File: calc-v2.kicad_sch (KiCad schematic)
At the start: 110 parts, among them IC1 ISL91107IRTNZ-T, J1 USB_C_Receptacle_USB2.0_16P, J2 Conn_01x02_MountingPin, SW1 SW_Push_45deg, SW10 SW_Push_45deg, SW11 SW_Push_45deg, SW12 SW_Push_45deg, SW13 SW_Push_45deg, SW14 SW_Push_45deg, SW15 SW_Push_45deg, SW16 SW_Push_45deg, SW17 SW_Push_45deg, SW18 SW_Push_45deg, SW19 SW_Push_45deg, SW2 SW_Push_45deg, SW20 SW_Push_45deg, SW21 SW_Push_45deg, SW22 SW_Push_45deg, SW23 SW_Push_45deg, SW24 SW_Push_45deg, SW25 SW_Push_45deg, SW26 SW_Push_45deg, SW27 SW_Push_45deg, SW28 SW_Push_45deg, SW29 SW_Push_45deg, SW3 SW_Push_45deg, SW30 SW_Push_45deg, SW31 SW_Push_45deg, SW32 SW_Push_45deg, SW33 SW_Push_45deg, SW34 SW_Push_45deg, SW35 SW_Push_45deg, SW36 SW_Push_45deg, SW37 SW_Push_45deg, SW38 SW_Push_45deg, SW39 SW_Push_45deg, SW4 SW_Push_45deg, SW40 SW_Push_45deg, SW41 SW_Push_45deg, SW42 SW_Push_45deg, SW43 SW_Push_45deg, SW44 SW_Push_45deg, SW45 SW_Push_45deg, SW46 SW_Push_45deg, SW47 SW_Push_45deg, SW48 SW_Push_45deg, SW49 SW_Push_45deg, SW5 SW_Push_45deg, SW6 SW_Push_45deg, SW7 SW_Push_45deg, SW8 SW_Push_45deg, SW9 SW_Push_45deg, U1 W25Q128JVS, U3 BQ24074RGT, U4 TPS61165DBV, U5 RP2350B, U6 APS6404L-3SQRx-ZR, Y1 ABM8-272-T3

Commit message: screen, moving buttons
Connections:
- net GND: now also DS1.3 (IM0), DS1.34 (DOTCLK), DS1.35 (ENABLE), DS1.4 (IM1), DS1.5 (IM2), DS1.6 (IM3)
- net RDX: now reaches U5.28 (GPIO27)
- net RDX: now also DS1.13 (~{RDX})
- net WRX: now reaches U5.36 (GPIO28)
- net WRX: now also DS1.12 (~{WRX})
- net DCX: now reaches U5.37 (GPIO29)
- net DCX: now also DS1.11 (DCX)
- net CSX: now reaches U5.38 (GPIO30)
- net CSX: now also DS1.10 (~{CSX})
- net DISPLAY_RESET: now reaches U5.39 (GPIO31)
- net DISPLAY_RESET: now also DS1.38 (~{RESX})
- net DB0: now reaches U5.40 (GPIO32)
- net DB0: now also DS1.14 (DB0)
- net DB1: now reaches U5.42 (GPIO33)
- net DB1: now also DS1.15 (DB1)
- net DB2: now reaches U5.43 (GPIO34)
- net DB2: now also DS1.16 (DB2)
- net DB3: now reaches U5.44 (GPIO35)
- net DB3: now also DS1.17 (DB3)
- net DB4: now reaches U5.45 (GPIO36)
- net DB4: now also DS1.18 (DB4)
- net DB5: now reaches U5.46 (GPIO37)
- net DB5: now also DS1.19 (DB5)
- net DB6: now reaches U5.47 (GPIO38)
- net DB6: now also DS1.20 (DB6)
- net DB7: now reaches U5.48 (GPIO39)
- net DB7: now also DS1.21 (DB7)
- no-connect marks 37 -> 39
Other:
- note added: "80-8bit parallel I/F"
- note added: "active low"
- moved on the sheet: C1, C10, C11, C12, C13, C14, C15, C16, C17, C2, C28, C29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

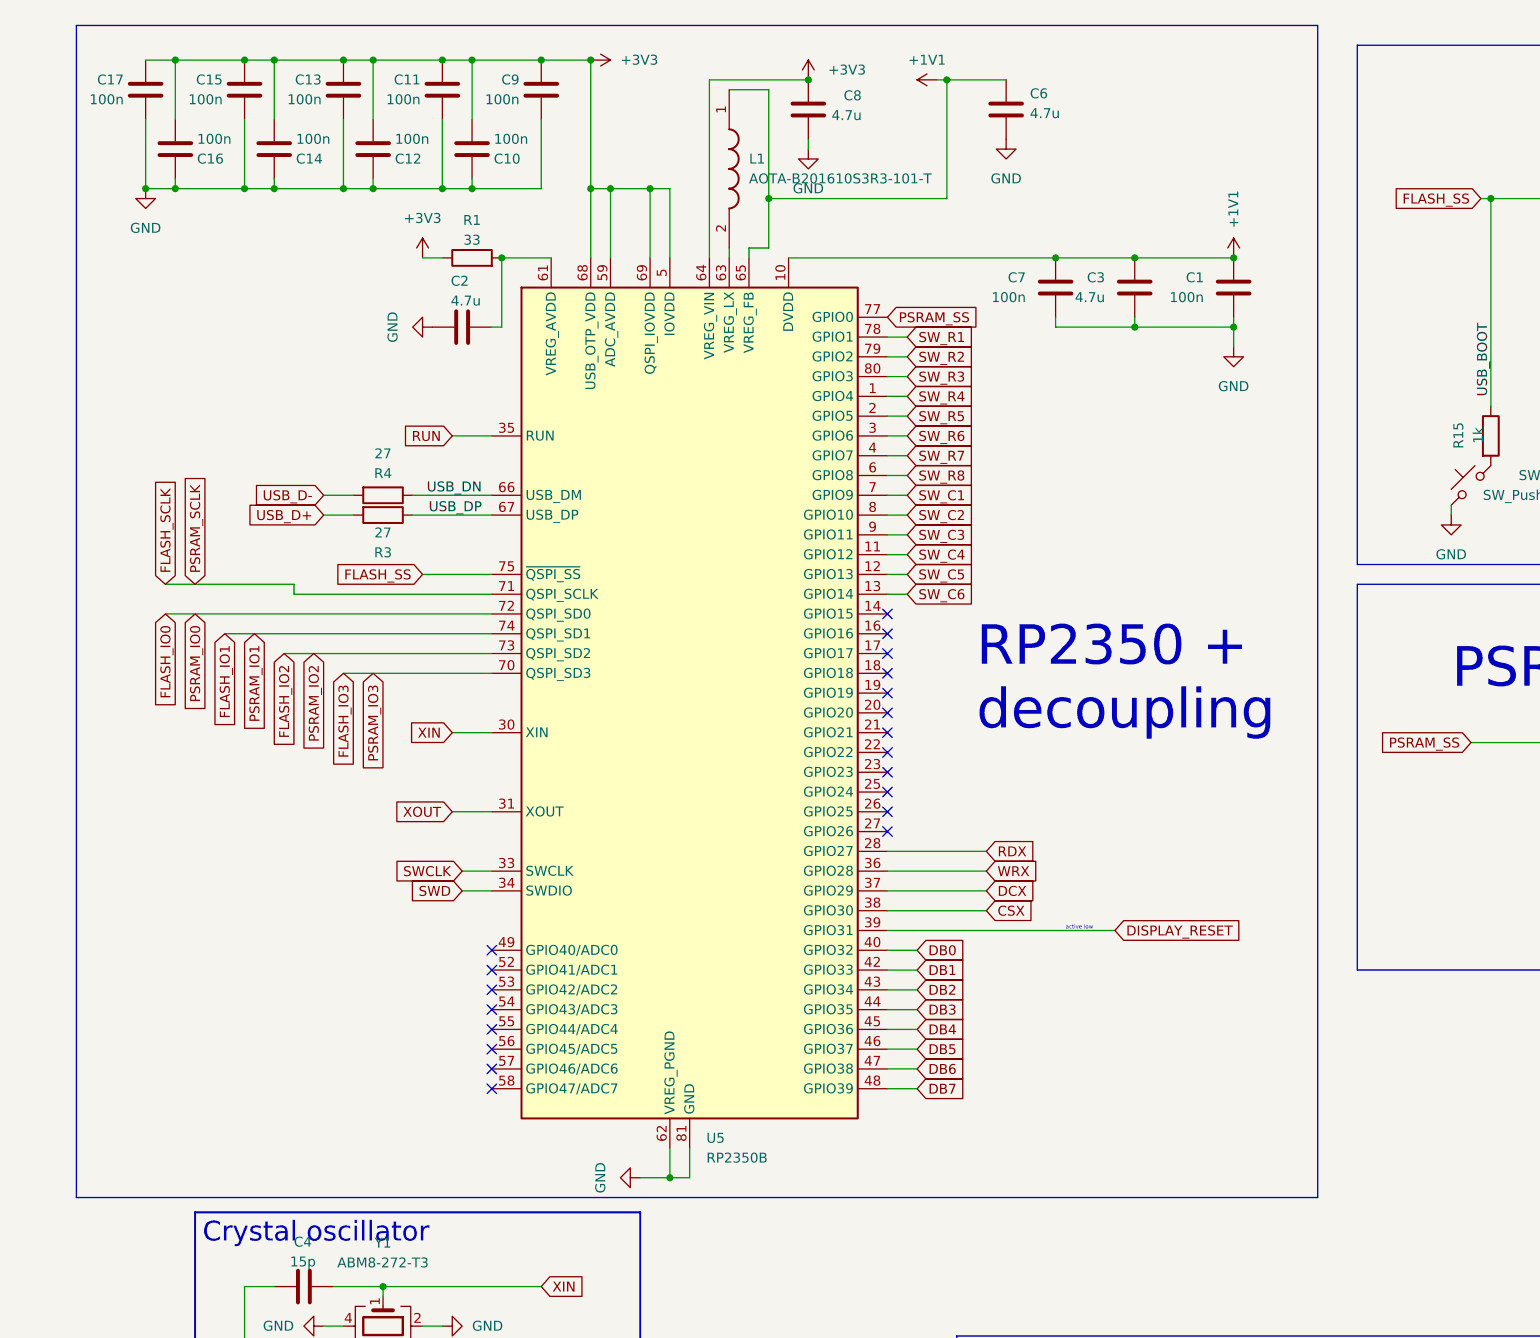
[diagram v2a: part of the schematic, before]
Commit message: more moving things
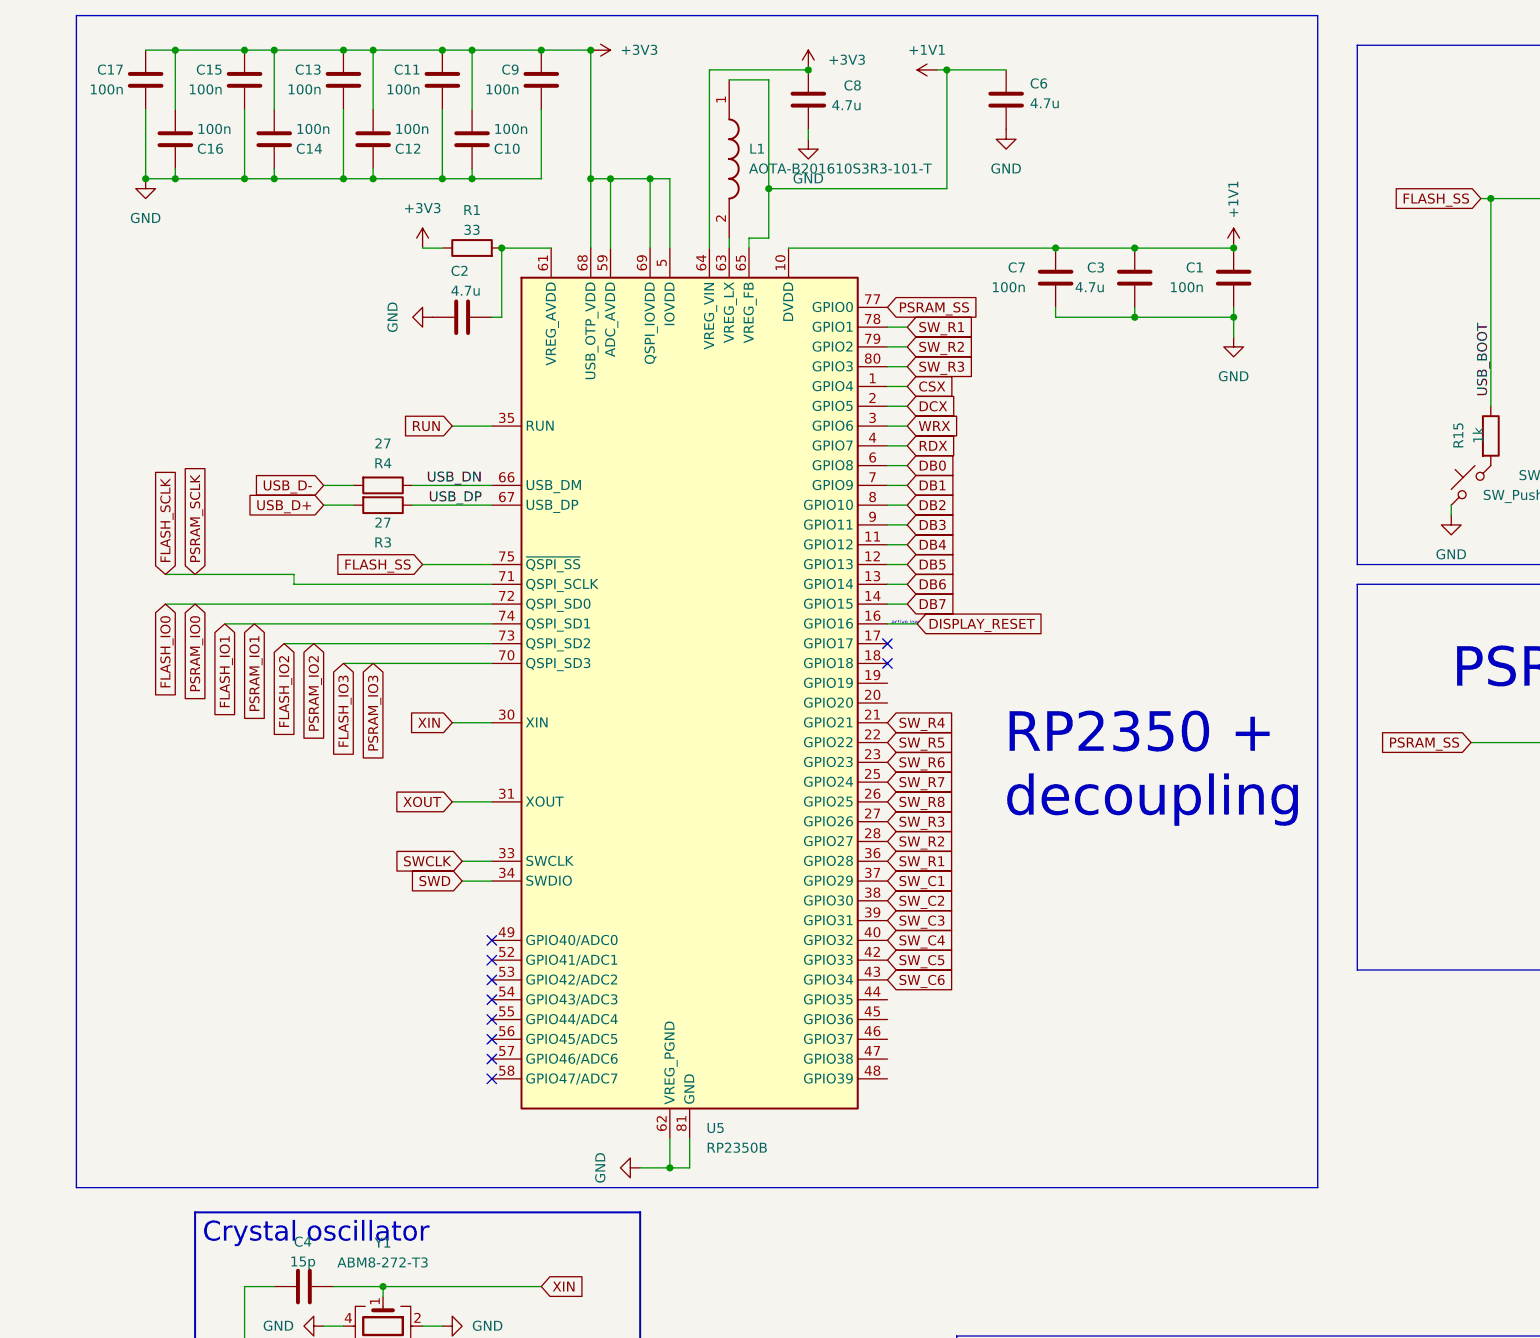
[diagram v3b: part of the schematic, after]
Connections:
- net CSX: now also U5.1 (GPIO4); no longer U5.38 (GPIO30)
- net DB0: now also U5.6 (GPIO8); no longer U5.40 (GPIO32)
- net DB1: now also U5.7 (GPIO9); no longer U5.42 (GPIO33)
- net DB2: now also U5.8 (GPIO10); no longer U5.43 (GPIO34)
- net DB3: now also U5.9 (GPIO11); no longer U5.44 (GPIO35)
- net DB4: now also U5.11 (GPIO12); no longer U5.45 (GPIO36)
- net DB5: now also U5.12 (GPIO13); no longer U5.46 (GPIO37)
- net DB6: now also U5.13 (GPIO14); no longer U5.47 (GPIO38)
- net DB7: now also U5.14 (GPIO15); no longer U5.48 (GPIO39)
- net DCX: now also U5.2 (GPIO5); no longer U5.37 (GPIO29)
- net DISPLAY_RESET: now also U5.16 (GPIO16); no longer U5.39 (GPIO31)
- net RDX: now also U5.4 (GPIO7); no longer U5.28 (GPIO27)
- net SW_C1: now also U5.37 (GPIO29); no longer U5.7 (GPIO9)
- net SW_C2: now also U5.38 (GPIO30); no longer U5.8 (GPIO10)
- net SW_C3: now also U5.39 (GPIO31); no longer U5.9 (GPIO11)
- net SW_C4: now also U5.40 (GPIO32); no longer U5.11 (GPIO12)
- net SW_C5: now also U5.42 (GPIO33); no longer U5.12 (GPIO13)
- net SW_C6: now also U5.43 (GPIO34); no longer U5.13 (GPIO14)
- net SW_R1: now also U5.36 (GPIO28)
- net SW_R2: now also U5.28 (GPIO27)
- net SW_R3: now also U5.27 (GPIO26)
- net SW_R4: now also U5.21 (GPIO21); no longer U5.1 (GPIO4)
- net SW_R5: now also U5.22 (GPIO22); no longer U5.2 (GPIO5)
- net SW_R6: now also U5.23 (GPIO23); no longer U5.3 (GPIO6)
- net SW_R7: now also U5.25 (GPIO24); no longer U5.4 (GPIO7)
- net SW_R8: now also U5.26 (GPIO25); no longer U5.6 (GPIO8)
- net WRX: now also U5.3 (GPIO6); no longer U5.36 (GPIO28)
- no-connect marks 39 -> 29
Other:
- moved on the sheet: C1, C10, C11, C12, C13, C14, C15, C16, C17, C2, C3, C6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
